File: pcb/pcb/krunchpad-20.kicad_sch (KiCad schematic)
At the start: 43 parts, among them J1 Conn_01x04_Socket, J2 Conn_01x04_Socket, SW1 SW_Push_45deg, SW10 SW_Push_45deg, SW11 SW_Push_45deg, SW12 SW_Push_45deg, SW13 SW_Push_45deg, SW14 SW_Push_45deg, SW15 SW_Push_45deg, SW16 SW_Push_45deg, SW17 SW_Push_45deg, SW18 SW_Push_45deg, SW19 SW_Push_45deg, SW2 SW_Push_45deg, SW20 SW_Push_45deg, SW3 SW_Push_45deg, SW4 SW_Push_45deg, SW5 SW_Push_45deg, SW6 SW_Push_45deg, SW7 SW_Push_45deg, SW8 SW_Push_45deg, SW9 SW_Push_45deg, U1 XIAO-RP2040-DIP

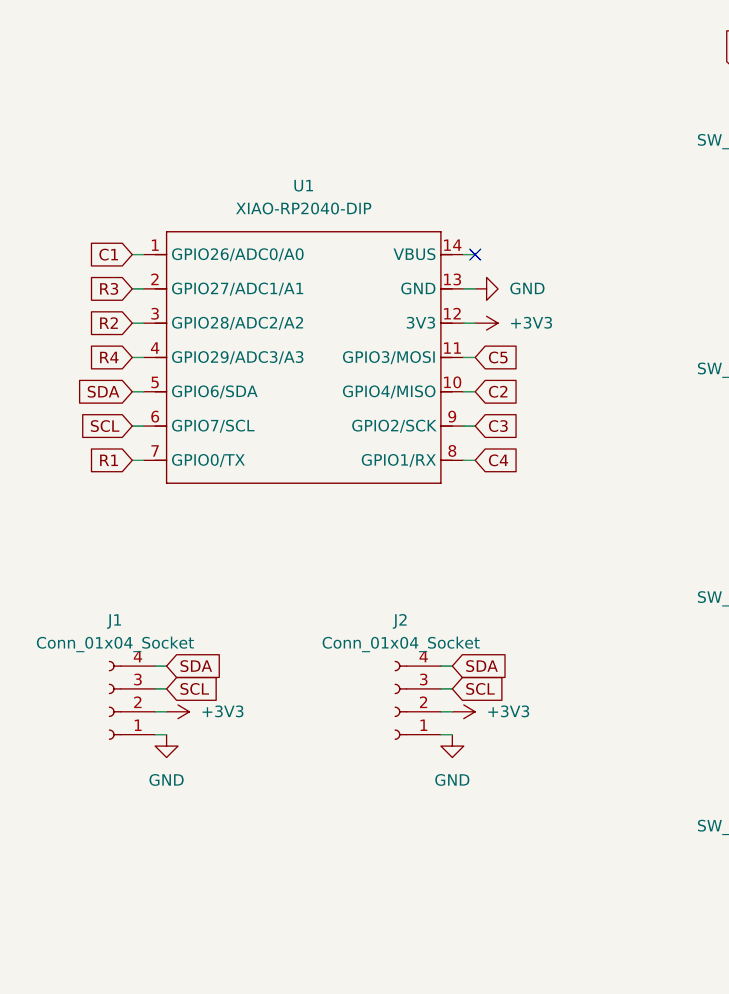
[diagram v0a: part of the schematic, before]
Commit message: updated pcb file with rotary encoder, updated gerber and case
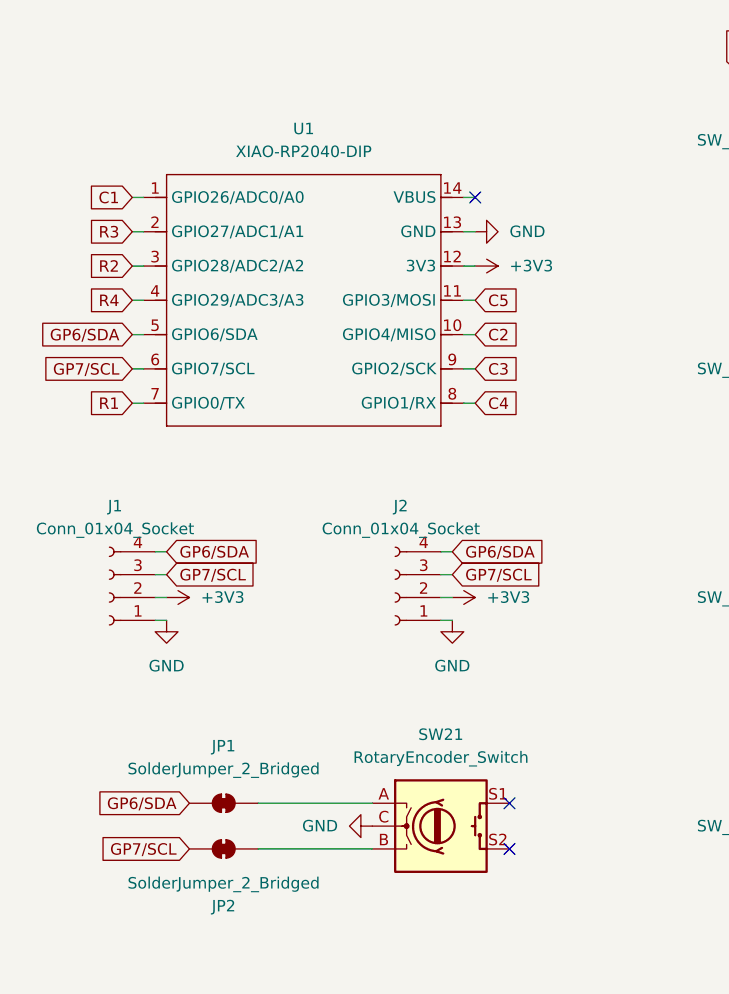
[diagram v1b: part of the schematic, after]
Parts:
- added JP1, JP2: SolderJumper_2_Bridged, Jumper:SolderJumper-2_P1.3mm_Bridged_RoundedPad1.0x1.5mm, symbol Jumper:SolderJumper_2_Bridged
- added SW21: RotaryEncoder_Switch, Rotary_Encoder:RotaryEncoder_Alps_EC11E-Switch_Vertical_H20mm, symbol Device:RotaryEncoder_Switch
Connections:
- net GND: now also SW21.C
- net SCL renamed GP7/SCL
- net GP7/SCL: now also JP2.2 (B)
- net SDA renamed GP6/SDA
- net GP6/SDA: now also JP1.1 (A)
- new net: JP2.1 (A), SW21.B
- new net: JP1.2 (B), SW21.A
- no-connect marks 1 -> 3
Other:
- moved on the sheet: J1, J2, U1
